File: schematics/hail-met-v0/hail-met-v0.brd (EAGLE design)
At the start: 77.1 x 61 mm, 110 parts, among them IC1 MCP73871, J1 AVR_SPI_PRG_6PTH, U1 ATMEGA328P, Y1 16MHZ

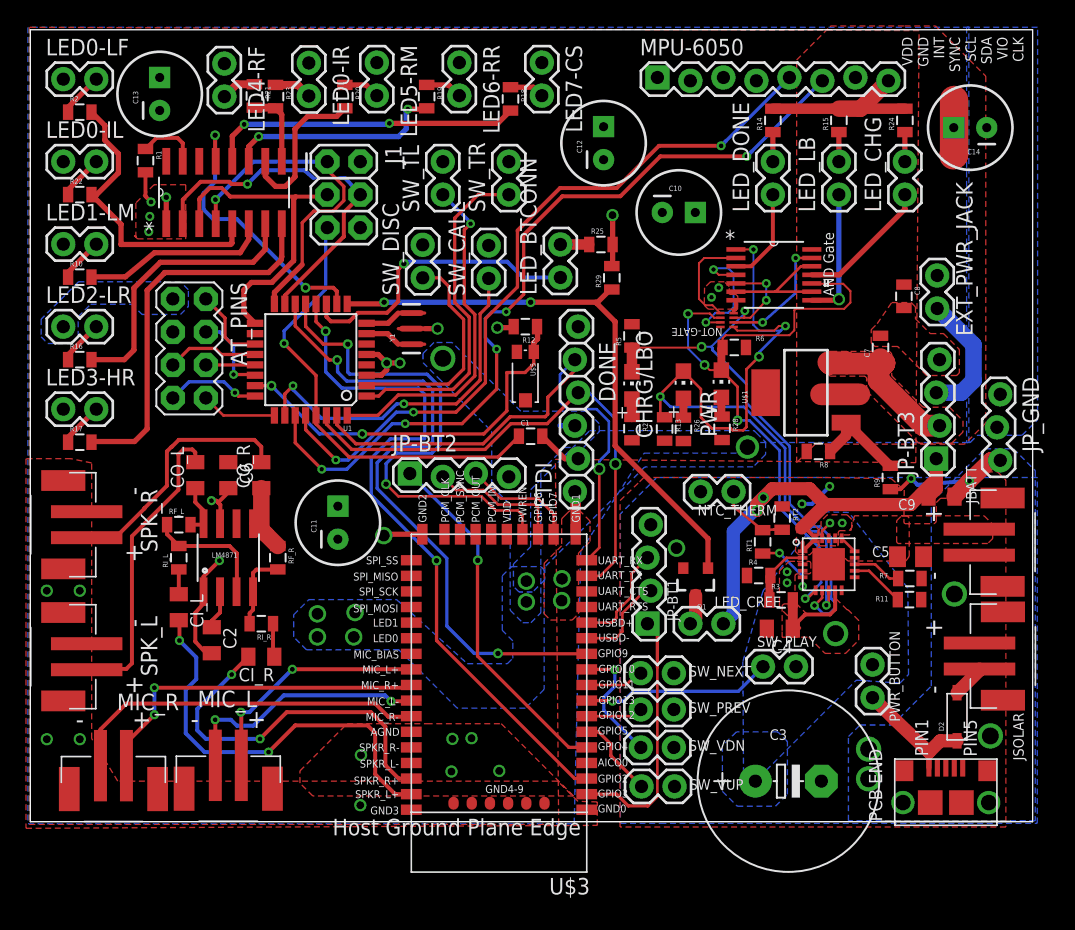
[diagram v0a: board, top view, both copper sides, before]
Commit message: ordered pcb
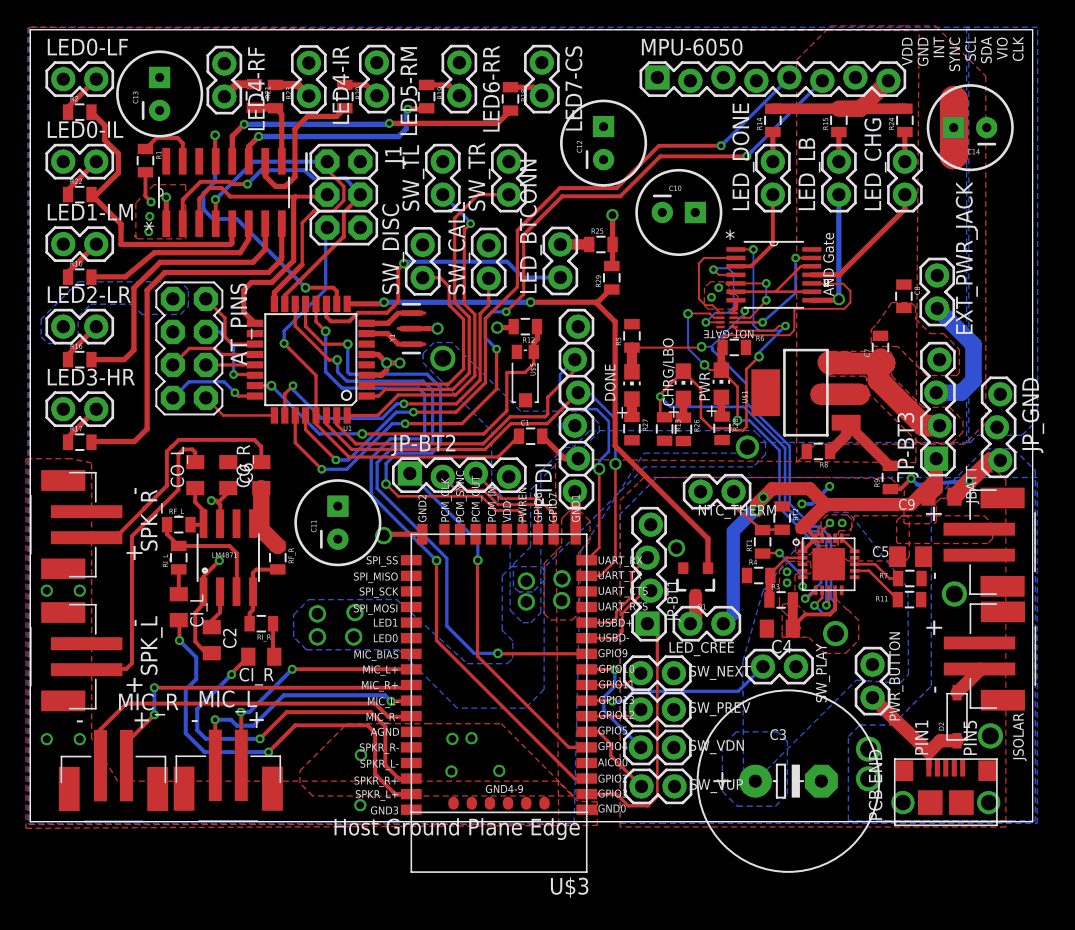
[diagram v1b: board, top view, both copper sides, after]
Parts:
- renumbered LED0-IR to LED4-IR
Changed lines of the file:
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@@
 <?xml version="1.0" encoding="utf-8"?>
 <!DOCTYPE eagle SYSTEM "eagle.dtd">
-<eagle version="7.1.0">
+<eagle version="6.5.0">
 <drawing>
 <settings>
@@
 <wire x1="77.14" y1="60.95" x2="0" y2="60.95" width="0" layer="20"/>
 <wire x1="0" y1="60.95" x2="0" y2="0" width="0" layer="20"/>
-<dimension x1="0" y1="60.95" x2="77.14" y2="60.95" x3="38.57" y3="68.58" textsize="1.778" layer="21" unit="inch"/>
-<dimension x1="77.14" y1="60.95" x2="77.47" y2="0" x3="100.157453125" y3="30.59873125" textsize="1.778" layer="21" unit="inch"/>
+<dimension x1="0" y1="60.95" x2="77.14" y2="60.95" x3="38.57" y3="68.58" textsize="1.778" layer="19" unit="inch"/>
+<dimension x1="77.14" y1="60.95" x2="77.47" y2="0" x3="100.157453125" y3="30.59873125" textsize="1.778" layer="19" unit="inch"/>
 <text x="67.0814" y="60.4012" size="0.8128" layer="25" rot="R90" align="top-right">VDD
 GND
@@
 <pass name="Default">
 <param name="RoutingGrid" value="50mil"/>
-<param name="AutoGrid" value="1"/>
-<param name="Efforts" value="0"/>
-<param name="TopRouterVariant" value="1"/>
 <param name="tpViaShape" value="round"/>
 <param name="PrefDir.1" value="|"/>
@@
 <element name="C8" library="SparkFun-Passives" package="0805" value="22pF" x="67.2338" y="40.4368" rot="R270"/>
 <element name="CHRG/LBO" library="adafruit" package="CHIP-LED0805" value="ORANGE" x="50.2666" y="33.6296" smashed="yes">
-<attribute name="NAME" x="47.879" y="29.5148" size="1.27" layer="25" rot="R90"/>
+<attribute name="NAME" x="49.5046" y="31.9532" size="0.8128" layer="25" rot="R90"/>
 </element>
 <element name="DONE" library="adafruit" package="CHIP-LED0805" value="GREEN" x="46.3042" y="33.5788" smashed="yes">
-<attribute name="NAME" x="45.0342" y="32.3088" size="1.27" layer="25" rot="R90"/>
+<attribute name="NAME" x="45.0342" y="32.3088" size="0.8128" layer="25" rot="R90"/>
 </element>
 <element name="FTDI" library="SparkFun-Connectors" package="1X06_LOCK" value="" x="41.91" y="25.4" rot="R90"/>
 <element name="IC1" library="adafruit" package="QFN20" value="MCP73871" x="61.4426" y="19.812" smashed="yes"/>
 <element name="LED_CREE" library="SparkFun-Connectors" package="1X02" value="M02PTH" x="53.34" y="15.24" smashed="yes" rot="R180">
-<attribute name="NAME" x="52.6542" y="16.51" size="0.8128" layer="25" ratio="10"/>
+<attribute name="NAME" x="49.0982" y="13.0048" size="0.8128" layer="25" ratio="10"/>
 </element>
 <element name="LED0-IL" library="SparkFun-Connectors" package="1X02" value="M02PTH" x="2.54" y="50.8" smashed="yes">
 <attribute name="NAME" x="1.1938" y="52.6288" size="1.27" layer="25" ratio="10"/>
 </element>
-<element name="LED0-IR" library="SparkFun-Connectors" package="1X02" value="M02PTH" x="21.4376" y="58.3946" smashed="yes" rot="R270">
+<element name="LED4-IR" library="SparkFun-Connectors" package="1X02" value="M02PTH" x="21.4376" y="58.3946" smashed="yes" rot="R270">
 <attribute name="NAME" x="23.2664" y="59.7408" size="1.27" layer="25" ratio="10" rot="R270"/>
 </element>
@@
 </element>
 <element name="PWR" library="adafruit" package="CHIP-LED0805" value="RED" x="53.1876" y="33.7058" smashed="yes">
-<attribute name="NAME" x="52.832" y="29.6164" size="1.27" layer="25" rot="R90"/>
+<attribute name="NAME" x="52.2986" y="32.3342" size="0.8128" layer="25" rot="R90"/>
 </element>
 <element name="R1" library="SparkFun-Passives" package="0805" value="" x="8.8646" y="50.8762" smashed="yes" rot="R270">
@@
 <attribute name="PROD_ID" value="XTAL-08900" x="29.337" y="37.9476" size="1.778" layer="27" rot="R90" display="off"/>
 </element>
-<element name="U$3" library="RN52" package="RN52" value="RN52" x="42.8244" y="22.1234" rot="R180">
+<element name="U$3" library="RN52" package="RN52" value="RN52" x="42.8244" y="22.1234" smashed="yes" rot="R180">
 <attribute name="DIGIKEY_OC" value="RN52-I/RM-ND" x="42.8244" y="22.1234" size="1.778" layer="27" rot="R180" display="off"/>
+<attribute name="NAME" x="43.0744" y="-4.3266" size="1.27" layer="21" rot="R180"/>
 </element>
 <element name="U$2" library="MicroUSB" package="10118193" value="10118193" x="70.4596" y="1.4732" smashed="yes">
@@
 </element>
 <element name="SW_PLAY" library="SparkFun-Connectors" package="1X02" value="M02PTH" x="56.388" y="11.938" smashed="yes">
-<attribute name="NAME" x="55.9308" y="13.462" size="0.8128" layer="25" ratio="10"/>
+<attribute name="NAME" x="61.2902" y="9.1186" size="0.8128" layer="25" ratio="10" rot="R90"/>
 </element>
 <element name="EXT_PWR_JACK" library="SparkFun-Connectors" package="1X02" value="M02PTH" x="69.7992" y="39.497" smashed="yes" rot="R90">
@@
 <attribute name="SUPPLIER" value="Texas Instruments" x="53.6194" y="38.608" size="1.778" layer="27" rot="R180" display="off"/>
 <attribute name="OC_FARNELL" value="-" x="53.6194" y="38.608" size="1.778" layer="27" rot="R180" display="off"/>
-<attribute name="NAME" x="53.2638" y="37.9984" size="0.6096" layer="25" ratio="10" rot="SR180"/>
+<attribute name="NAME" x="55.7276" y="37.8206" size="0.6096" layer="25" ratio="10" rot="SR180"/>
 </element>
 <element name="D2" library="adafruit" package="SOD-123" value="" x="71.3232" y="8.0772" rot="R90"/>
@@
 <contactref element="LED4-RF" pad="1"/>
 <contactref element="LED0-IL" pad="1"/>
-<contactref element="LED0-IR" pad="1"/>
+<contactref element="LED4-IR" pad="1"/>
 <contactref element="LM4871" pad="6"/>
 <contactref element="C6" pad="1"/>
@@
 </signal>
 <signal name="N$66">
-<contactref element="LED0-IR" pad="2"/>
+<contactref element="LED4-IR" pad="2"/>
 <contactref element="R23" pad="1"/>
 <wire x1="18.8722" y1="56.7038" x2="20.5884" y2="56.7038" width="0.6096" layer="1"/>
